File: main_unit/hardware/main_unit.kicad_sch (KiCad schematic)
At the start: 14 parts, among them SW1 SW_SPST, U1 STM32H753ZIT6, Y1 ABM8G-25.000MHZ-18-D2Y-T, Y2 SC32S-7PF20PPM

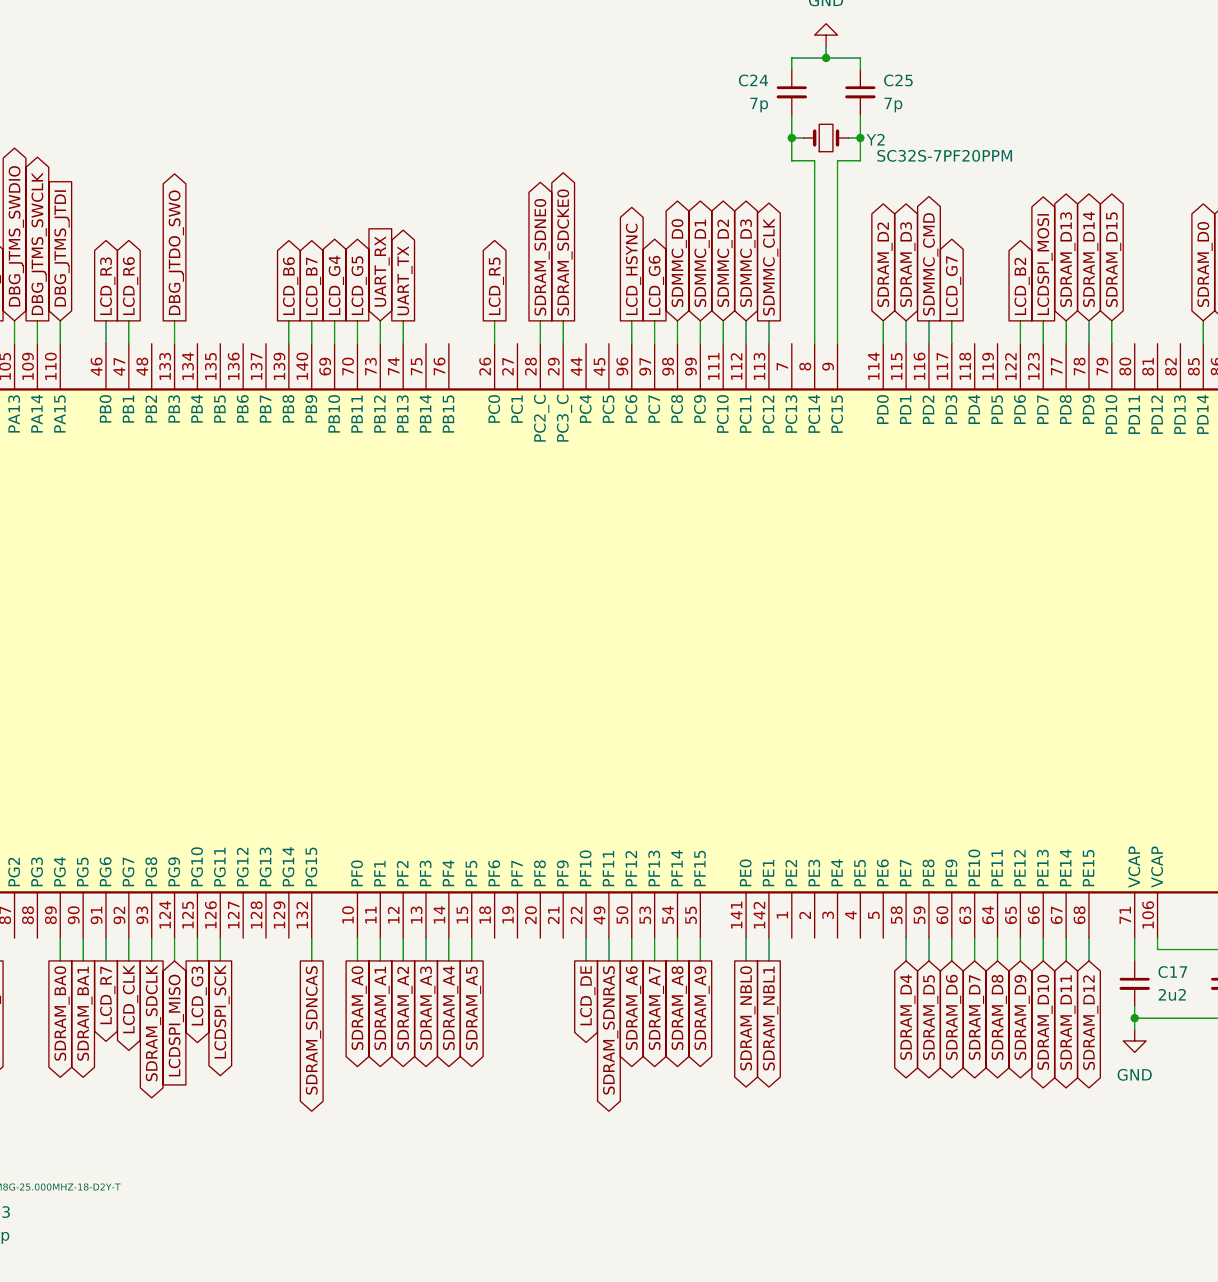
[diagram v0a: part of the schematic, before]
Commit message: main_unit/hardware: Add in display connector, expand LTDC to RGB888 (fixes pin error)
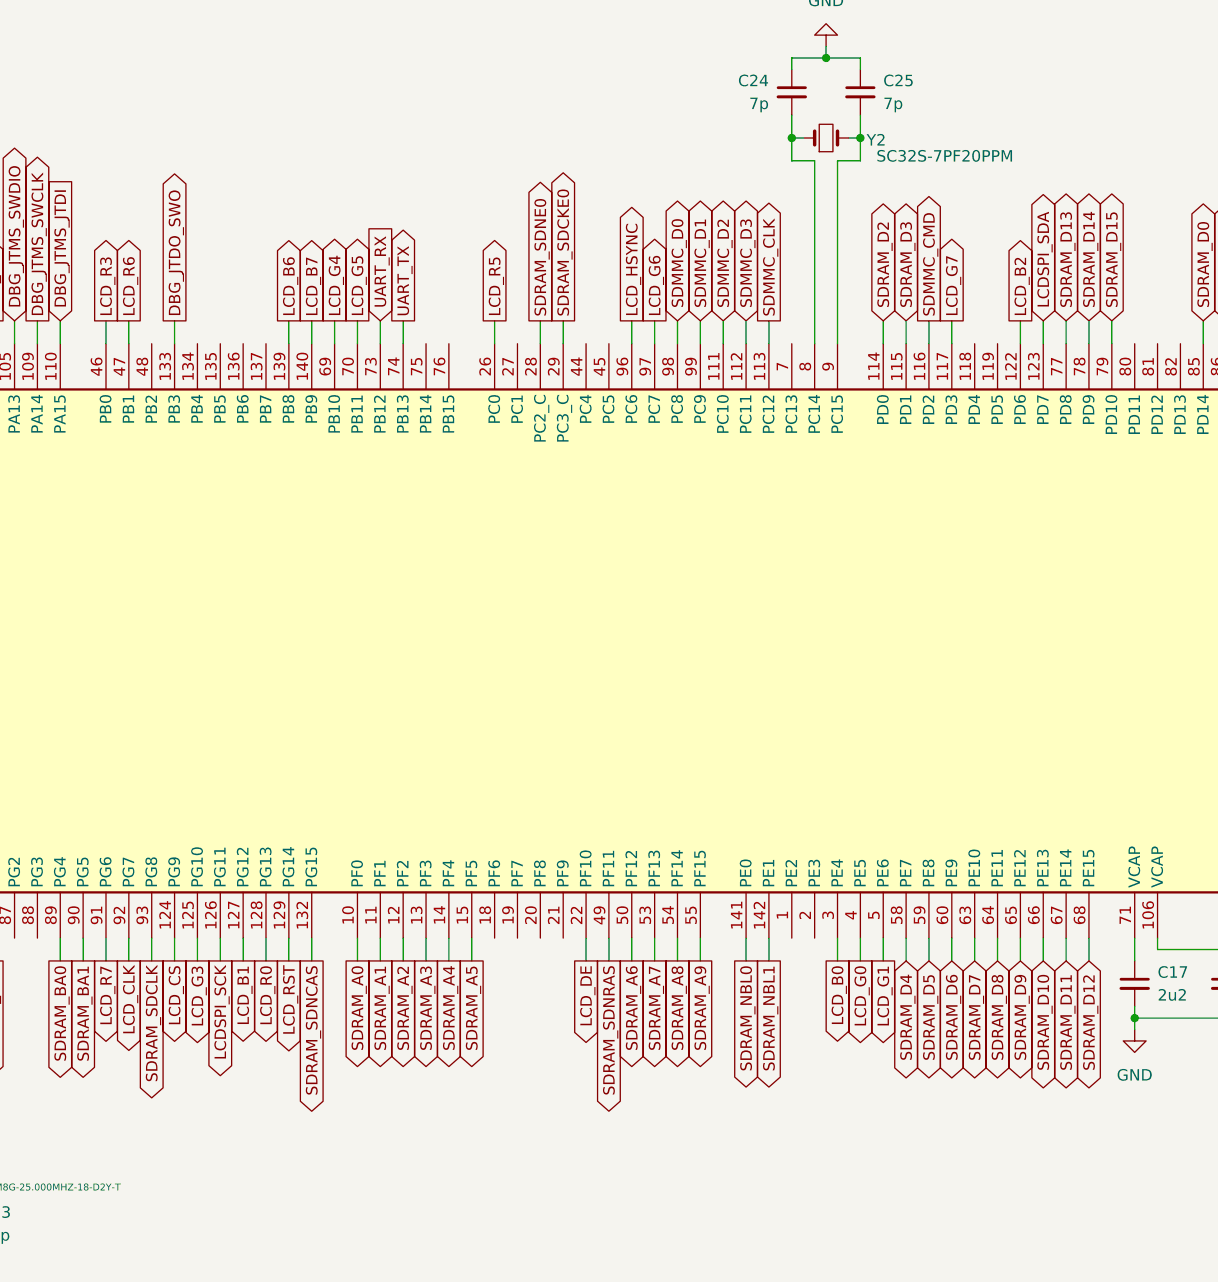
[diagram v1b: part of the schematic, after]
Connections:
- net LCD_B1: now reaches U1.127 (PG12)
- net LCD_R0: now reaches U1.128 (PG13)
- net LCD_RST: now reaches U1.129 (PG14)
- net LCD_B0: now reaches U1.3 (PE4)
- net LCD_G0: now reaches U1.4 (PE5)
- net LCD_G1: now reaches U1.5 (PE6)
- net LCDSPI_MISO renamed LCD_CS
- net LCDSPI_MOSI renamed LCDSPI_SDA

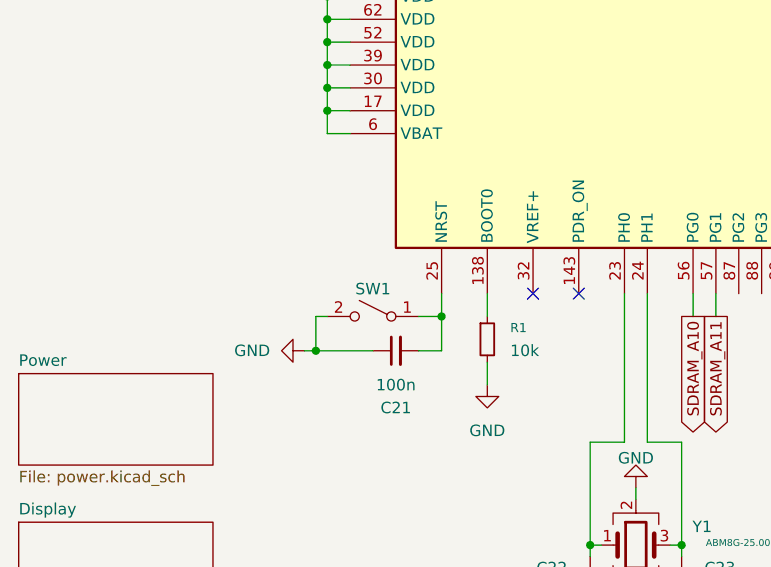
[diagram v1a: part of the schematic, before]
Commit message: main_unit/hardware: Change reset button type
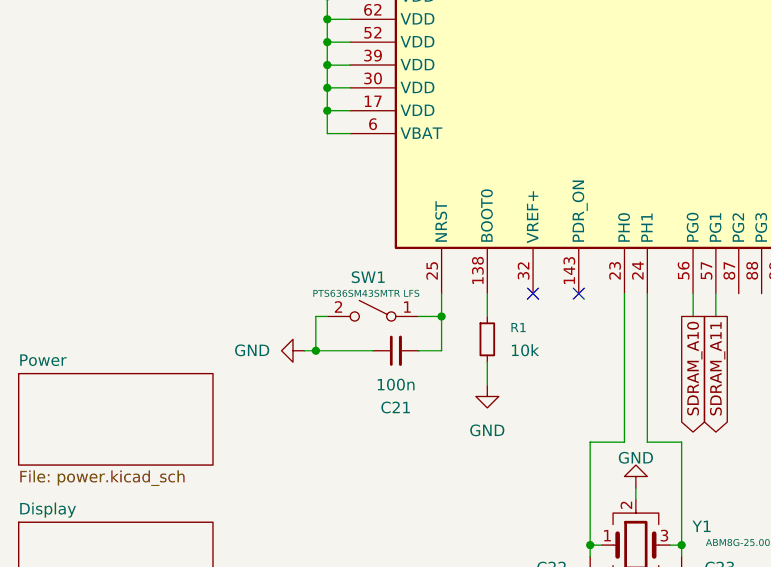
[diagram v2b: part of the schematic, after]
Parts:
- SW1: value SW_SPST -> PTS636SM43SMTR LFS; footprint Connector_PinHeader_2.54mm:PinHeader_1x02_P2.54mm_Vertical -> Button_Switch_SMD:SW_Tactile_SPST_NO_Straight_CK_PTS636Sx25SMTRLFS
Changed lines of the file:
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@@
 		(dnp no)
 		(property "Reference" "SW1"
-			(at 54.61 125.222 0)
+			(at 54.102 123.952 0)
 			(effects
 				(font
@@
 			)
 		)
-		(property "Value" "SW_SPST"
-			(at 54.61 124.46 0)
+		(property "Value" "PTS636SM43SMTR LFS"
+			(at 53.848 125.73 0)
 			(effects
 				(font
-					(size 1.27 1.27)
+					(size 0.762 0.762)
 				)
-				(hide yes)
 			)
 		)
-		(property "Footprint" "Connector_PinHeader_2.54mm:PinHeader_1x02_P2.54mm_Vertical"
+		(property "Footprint" "Button_Switch_SMD:SW_Tactile_SPST_NO_Straight_CK_PTS636Sx25SMTRLFS"
 			(at 54.61 128.27 0)
 			(effects

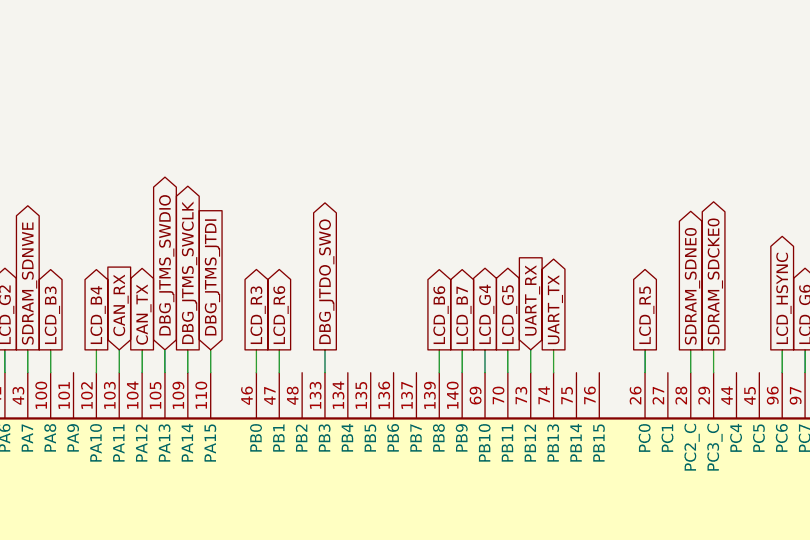
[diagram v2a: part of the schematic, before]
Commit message: main_unit/hardware: Connect LCD controller FAULT and PWM pin to STM32
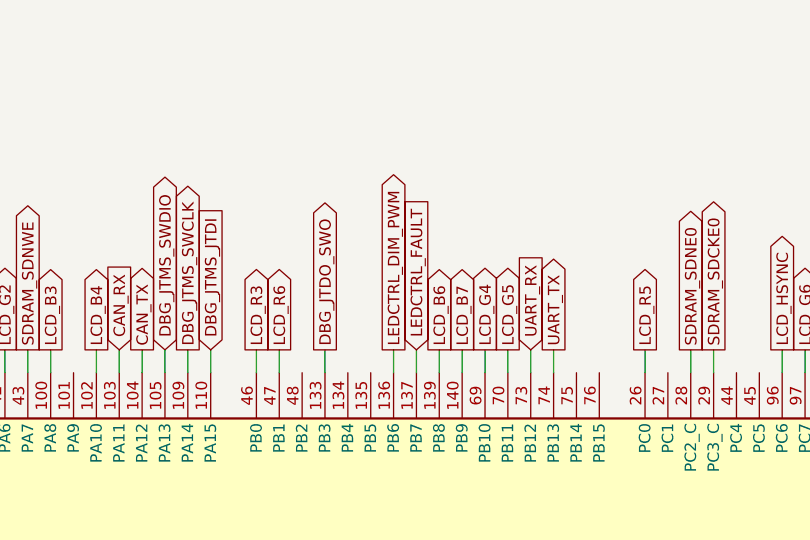
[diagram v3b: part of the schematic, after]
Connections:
- net LEDCTRL_DIM_PWM: now reaches U1.136 (PB6)
- net LEDCTRL_FAULT: now reaches U1.137 (PB7)
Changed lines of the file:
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@@
+	(wire
+		(pts
+			(xy 123.19 57.15) (xy 123.19 59.69)
+		)
+		(stroke
+			(width 0)
+			(type default)
+		)
+	)
 	(wire
 		(pts
@@
 		(pts
 			(xy 49.53 74.93) (xy 49.53 77.47)
+		)
+		(stroke
+			(width 0)
+			(type default)
+		)
+	)
+	(wire
+		(pts
+			(xy 120.65 57.15) (xy 120.65 59.69)
 		)
 		(stroke
@@
 		)
 	)
+	(global_label "LEDCTRL_DIM_PWM"
+		(shape output)
+		(at 120.65 57.15 90)
+		(fields_autoplaced yes)
+		(effects
+			(font
+				(size 1.27 1.27)
+			)
+			(justify left)
+		)
+		(property "Intersheetrefs" "${INTERSHEET_REFS}"
+			(at 120.65 36.7478 90)
+			(effects
+				(font
+					(size 1.27 1.27)
+				)
+				(justify left)
+				(hide yes)
+			)
+		)
+	)
 	(global_label "SDRAM_BA1"
 		(shape output)
@@
 				(hide yes)
 			)
+		)
+	)
+	(global_label "LEDCTRL_FAULT"
+		(shape input)
+		(at 123.19 57.15 90)
+		(fields_autoplaced yes)
+		(effects
+			(font
+				(size 1.27 1.27)
+			)
+			(justify left)
+		)
+		(property "Intersheetrefs" "${INTERSHEET_REFS}"
+			(at 123.19 39.711 90)
+			(effects
+				(font
+					(size 1.27 1.27)
+				)
+				(justify left)
+				(hide yes)
+			)
